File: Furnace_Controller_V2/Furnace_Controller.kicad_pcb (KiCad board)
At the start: 2 copper layers, 149 x 141 mm, 99 parts, among them J1 Power In Treminal, J3 Relay Terminal, J4 HMD Terminal, J5 RS-485 Terminal, Q1 IRLZ44N, Q2 IRLZ44N, Q3 IRLZ44N, Q4 IRLZ44N, Q5 2n2222, U2 LM2596S-5, U3 THVD2450DR, U4 TXU0101DBVR, U5 TXU0101DBVR, U6 TVS3300DRV

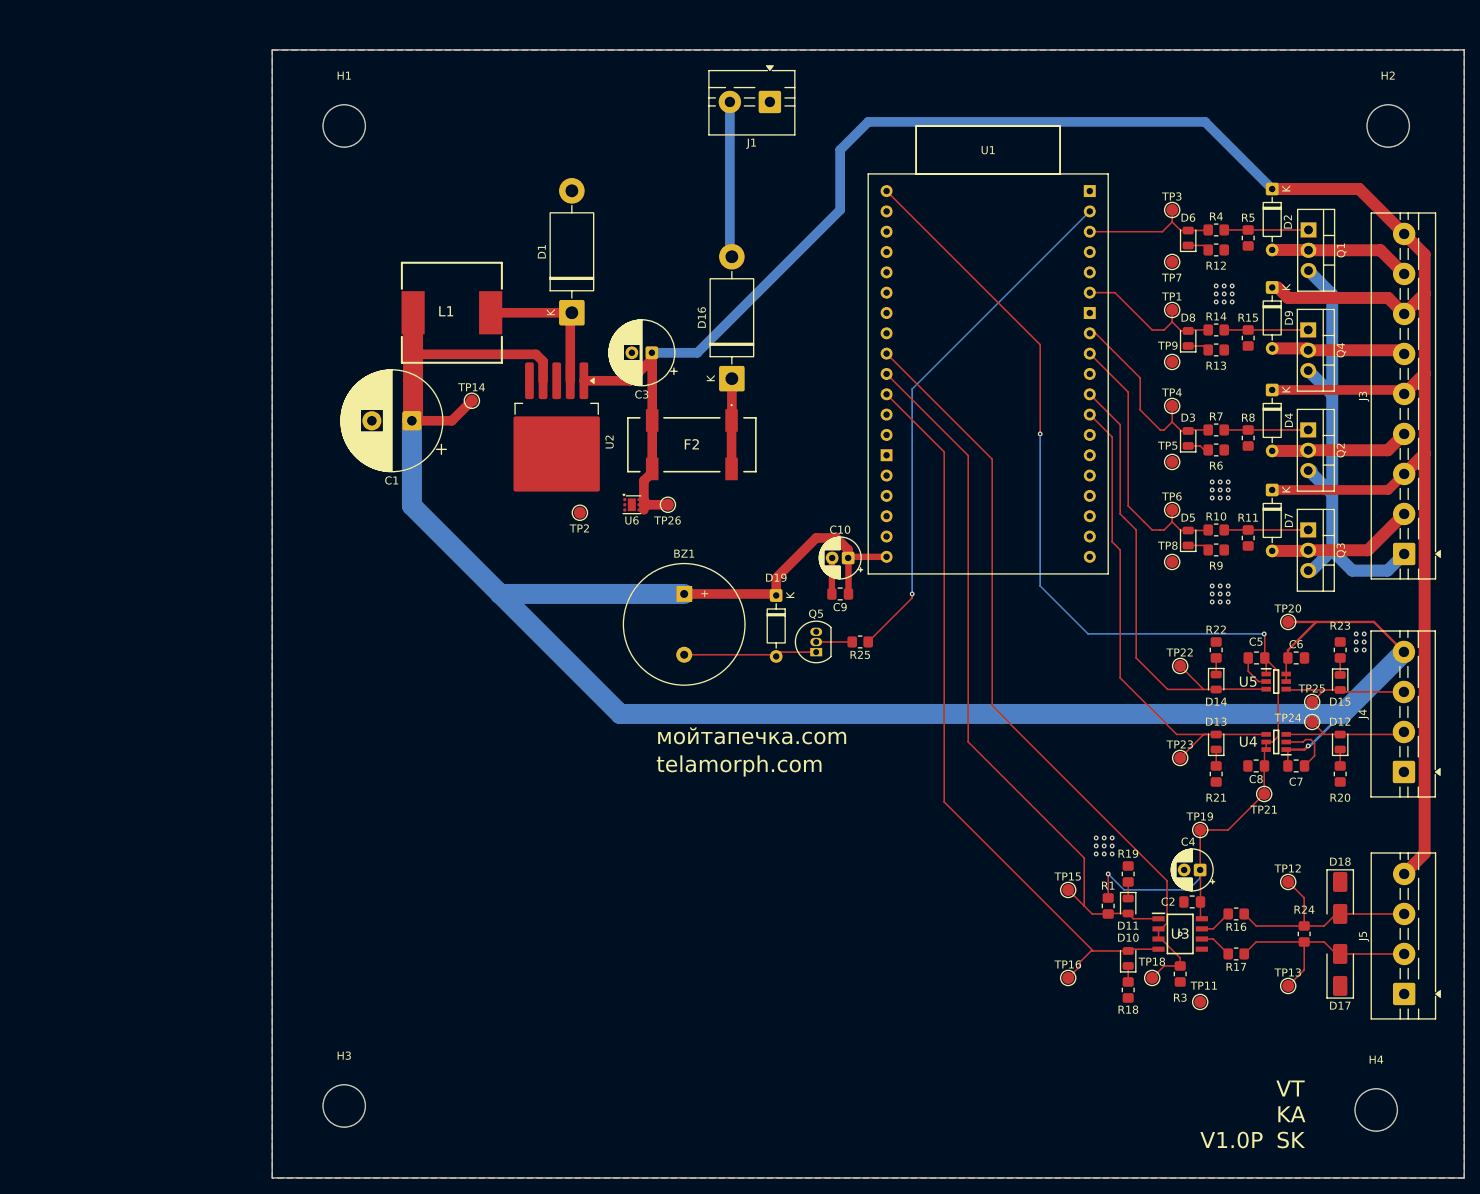
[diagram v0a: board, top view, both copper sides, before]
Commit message: V2 dev
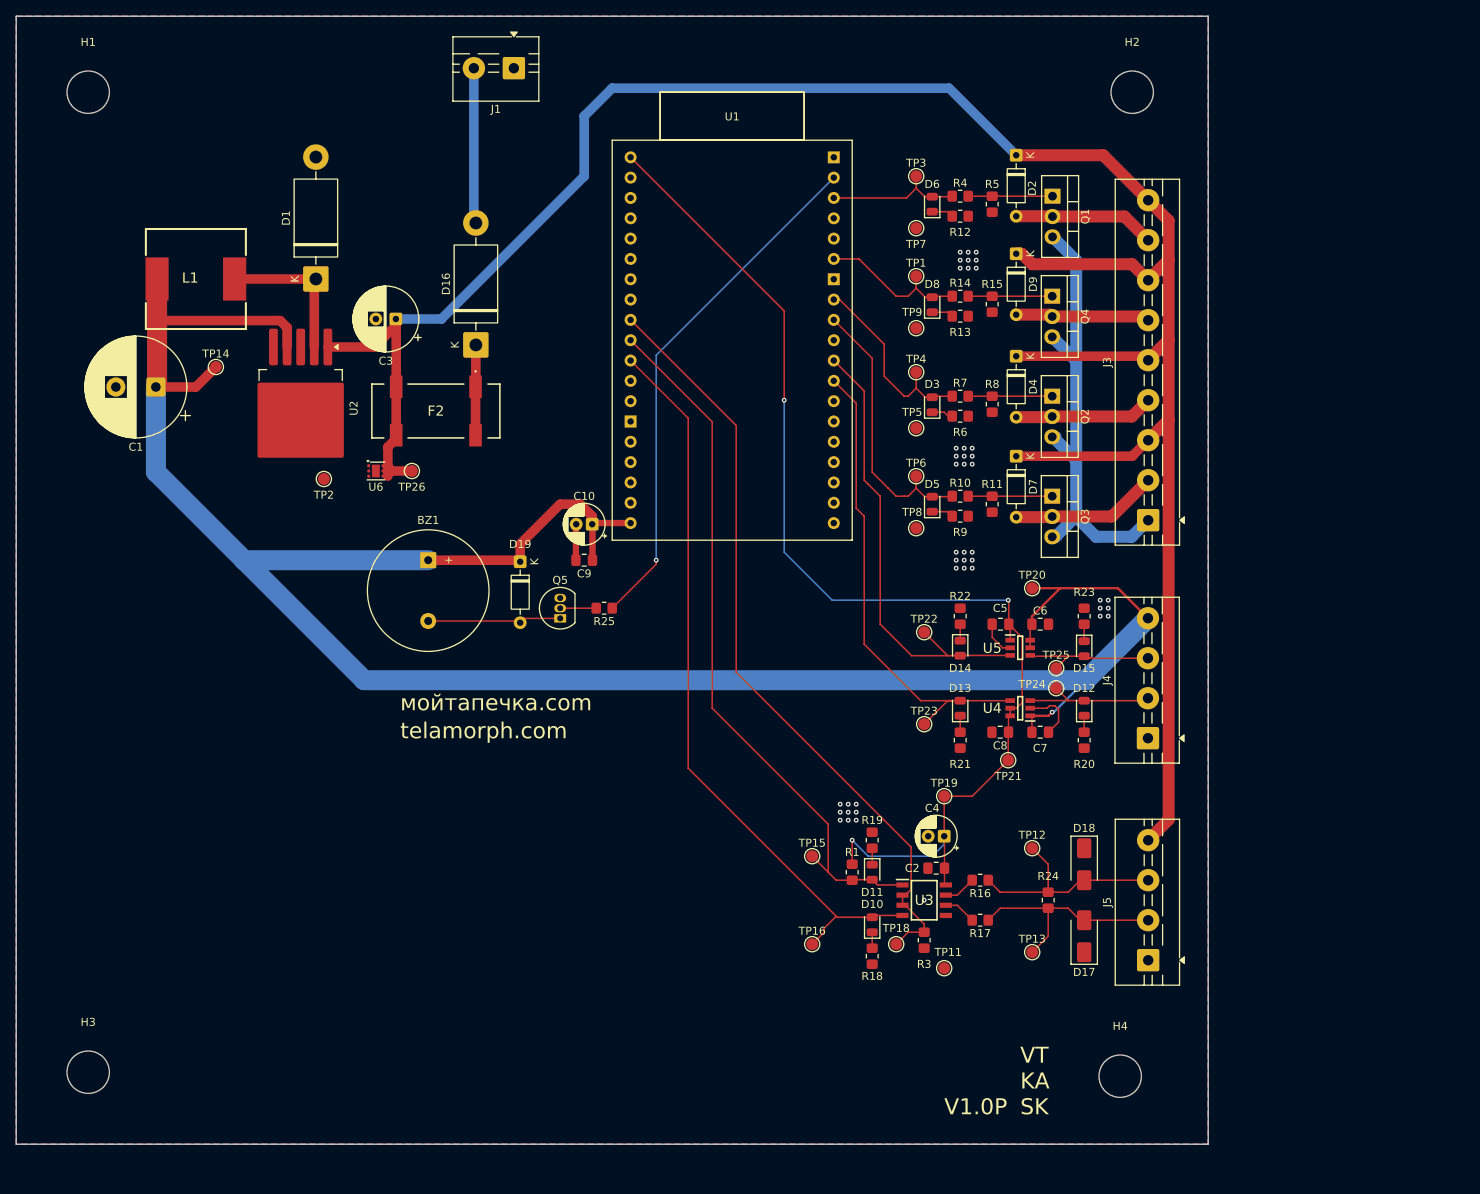
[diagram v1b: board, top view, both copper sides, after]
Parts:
- moved BZ1 32.3 mm to (68.5, 83.8)
- moved C10 32.3 mm to (89.0, 79.3)
- moved C2 32.3 mm to (132.0, 122.3)
- moved C3 32.3 mm to (64.5, 53.6)
- moved C4 32.3 mm to (133.0, 118.3)
- moved C5 32.3 mm to (140.0, 91.8)
- moved C6 32.3 mm to (145.0, 91.8)
- moved C7 32.3 mm to (145.0, 105.3)
- moved C8 32.3 mm to (140.0, 105.3)
- moved C9 32.3 mm to (88.0, 83.8)
- moved D10 32.3 mm to (124.0, 129.3)
- moved D11 32.3 mm to (124.0, 122.8)
- moved D12 32.3 mm to (150.5, 102.3)
- moved D13 32.3 mm to (135.0, 102.3)
- moved D14 32.3 mm to (135.0, 94.8)
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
